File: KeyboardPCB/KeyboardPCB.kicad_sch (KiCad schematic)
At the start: 2 parts

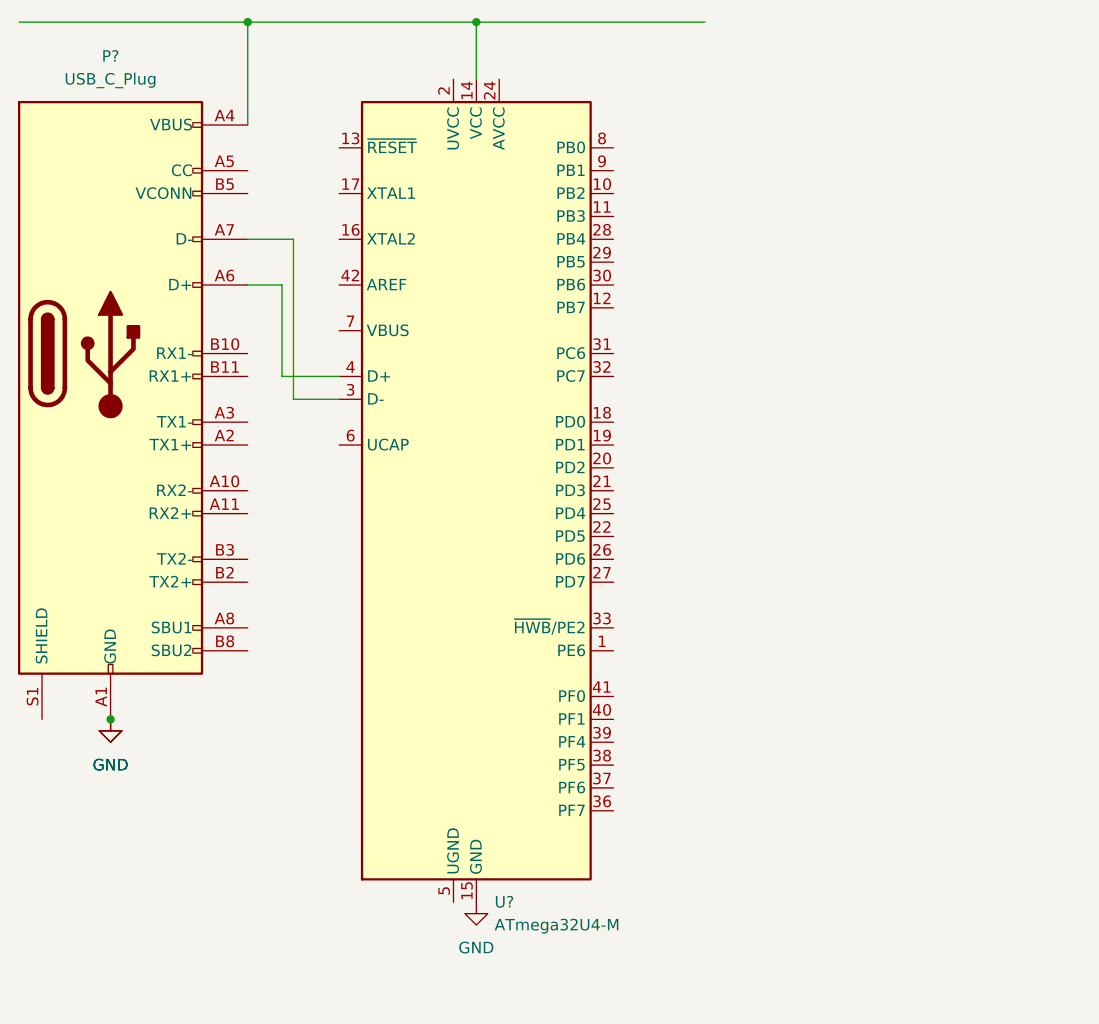
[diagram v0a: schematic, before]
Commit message: Made progress on keyboard schematic
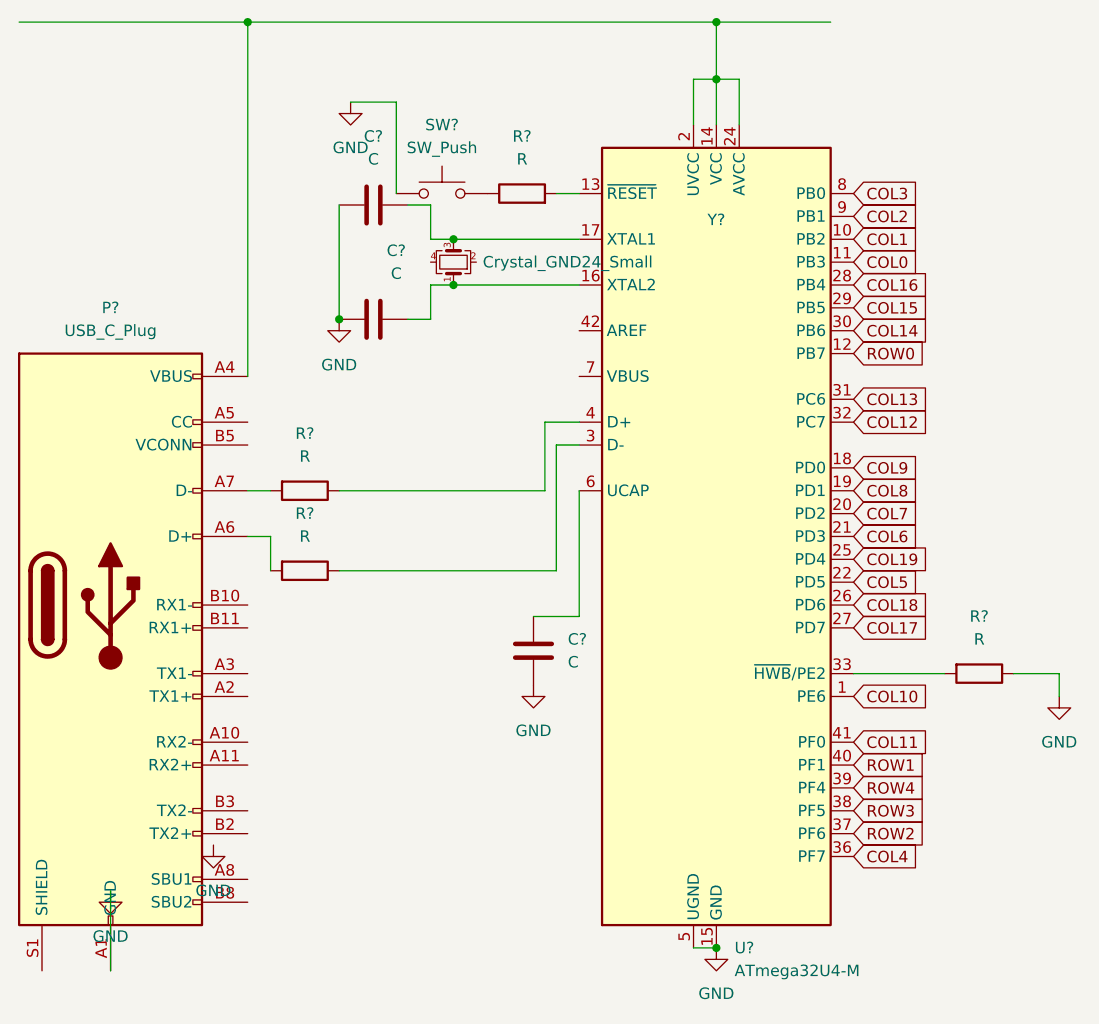
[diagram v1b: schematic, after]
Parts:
- added C? (x3): C, symbol Device:C
- added R? (x4): R, symbol Device:R
- added SW?: SW_Push, symbol Switch:SW_Push
- added Y?: Crystal_GND24_Small, symbol Device:Crystal_GND24_Small
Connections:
- net GND: now also U?.5 (UGND), C?.2, C?.2, C?.2, R?.1, SW?.1
- net at P?.A4 (VBUS), P?.A9 (VBUS), P?.B4 (VBUS)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: now also U?.2 (UVCC), U?.24 (AVCC), U?.44 (AVCC)
- net at U?.4 (D+): now also R?.1; no longer P?.A6 (D+)
- net at P?.A7 (D-): now also R?.2; no longer U?.3 (D-)
- net COL10: now reaches U?.1 (PE6)
- net COL1: now reaches U?.10 (PB2)
- net COL0: now reaches U?.11 (PB3)
- net ROW0: now reaches U?.12 (PB7)
- net at U?.13 (~{RESET}): now also R?.2
- net at U?.16 (XTAL2): now also C?.1, Y?.1
- net at U?.17 (XTAL1): now also C?.1, Y?.3
- net COL9: now reaches U?.18 (PD0)
- net COL8: now reaches U?.19 (PD1)
- net COL7: now reaches U?.20 (PD2)
- net COL6: now reaches U?.21 (PD3)
- net COL5: now reaches U?.22 (PD5)
- net COL19: now reaches U?.25 (PD4)
- net COL18: now reaches U?.26 (PD6)
- net COL17: now reaches U?.27 (PD7)
- net COL16: now reaches U?.28 (PB4)
- net COL15: now reaches U?.29 (PB5)
- net COL14: now reaches U?.30 (PB6)
- net COL13: now reaches U?.31 (PC6)
- net COL12: now reaches U?.32 (PC7)
- net at U?.33 (~{HWB}/PE2): now also R?.2
- net COL4: now reaches U?.36 (PF7)
- net ROW2: now reaches U?.37 (PF6)
- net ROW3: now reaches U?.38 (PF5)
- net ROW4: now reaches U?.39 (PF4)
- net ROW1: now reaches U?.40 (PF1)
- net COL11: now reaches U?.41 (PF0)
- net at U?.6 (UCAP): now also C?.1
- net COL3: now reaches U?.8 (PB0)
- net COL2: now reaches U?.9 (PB1)
- new net: R?.1, SW?.2
- new net: P?.A6 (D+), R?.2
- new net: R?.1, U?.3 (D-)
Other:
- moved on the sheet: P?, U?
